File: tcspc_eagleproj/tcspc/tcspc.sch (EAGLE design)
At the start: 72 parts, among them U1 THS788, U2 MCP4725, U3 ADCMP582, U4 LT6003_SOT23-5, X1 SMA

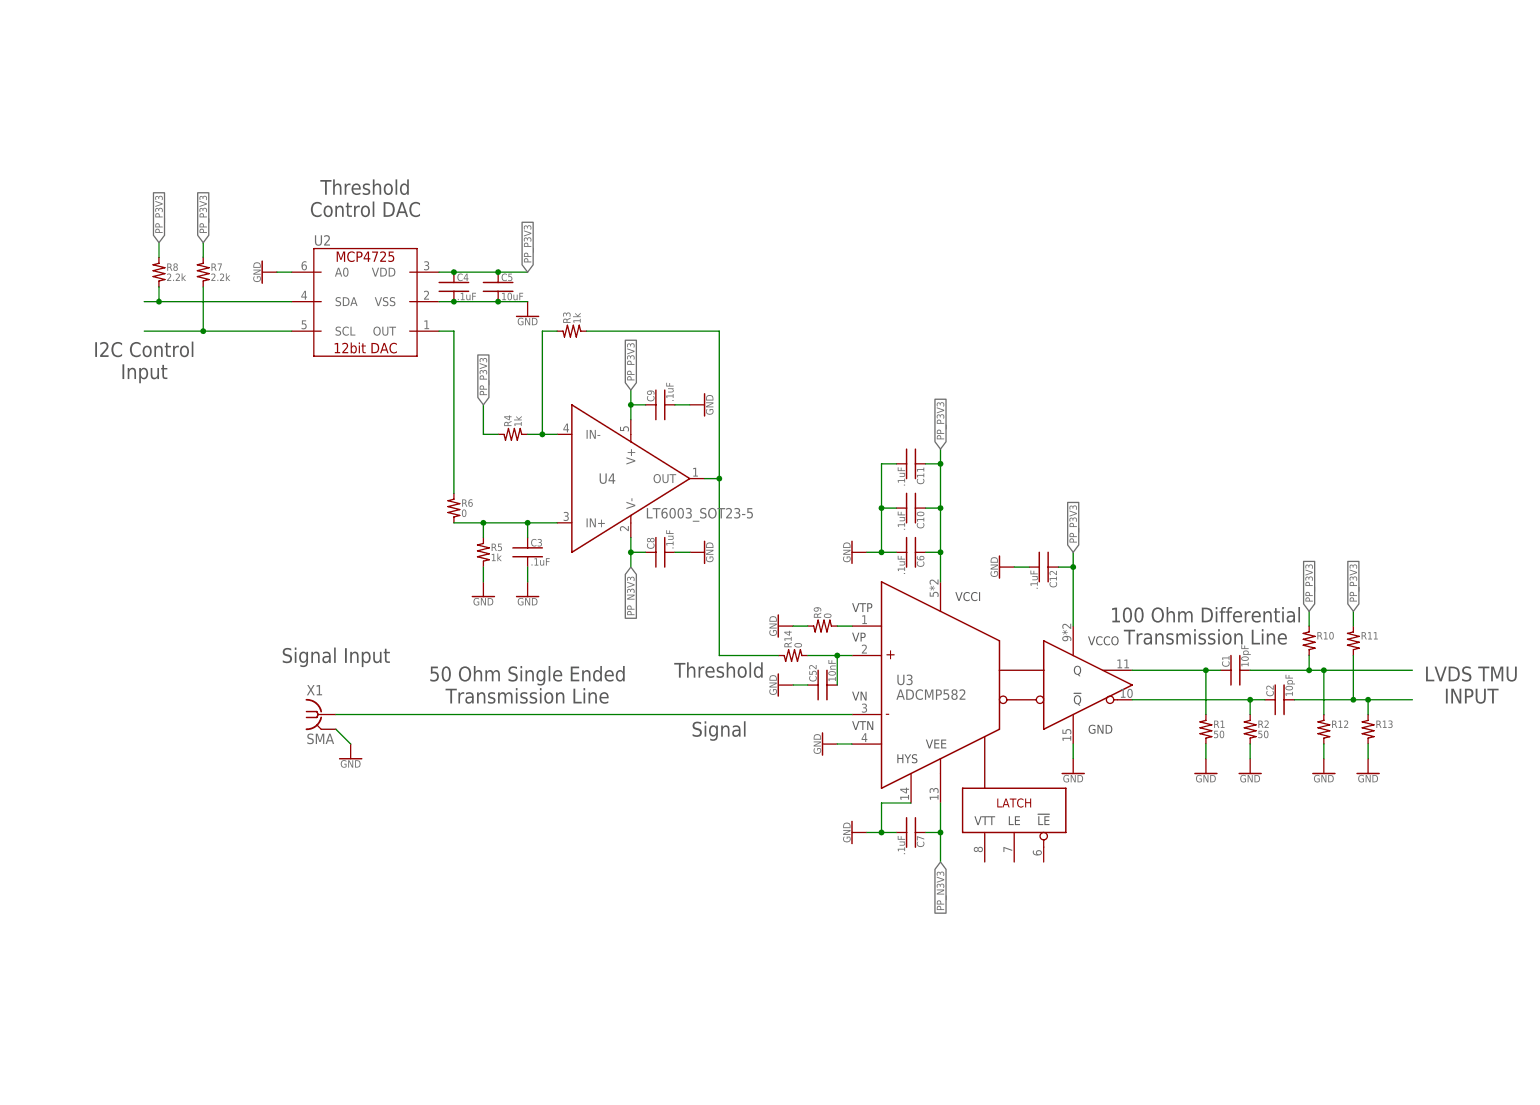
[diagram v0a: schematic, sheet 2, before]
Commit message: not 100% sure what changes got made here but there was a good chunk of progress nonetheless
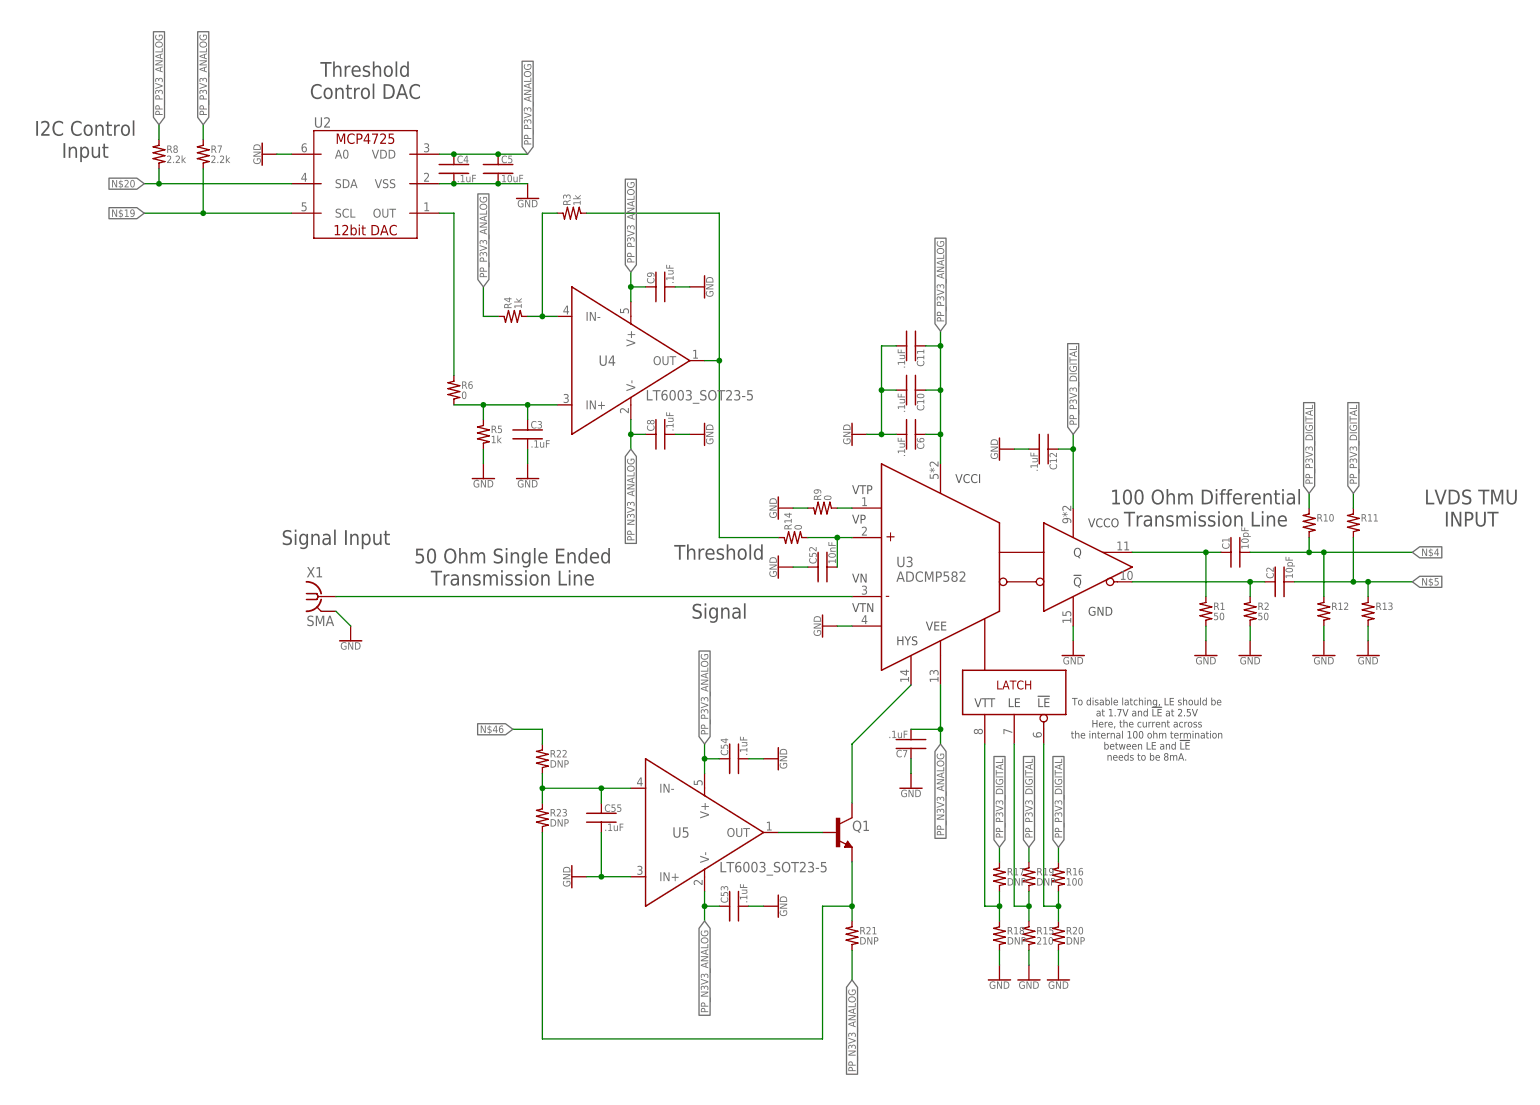
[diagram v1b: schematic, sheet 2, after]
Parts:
- added C53, C54, C55: .1uF, tcspc_lib:CAP_0402
- added Q1: (no value), jack_semi:BJT_NPN
- added R15: 210, tcspc_lib:RES_0402
- added R16: 100, tcspc_lib:RES_0402
- added R17, R18, R19, R20, R21, R22, R23: DNP, tcspc_lib:RES_0402
- added U5: LT6003_SOT23-5, tcspc_lib:LT6003_SOT23-5
- C3, C4, C5, C8, C9: device tcspc_lib:CAP_0603 -> tcspc_lib:CAP_0402
- R3, R4, R5, R6, R7, R8: device tcspc_lib:RES_0603 -> tcspc_lib:RES_0402
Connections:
- removed net PP_N3V3: C7.1, C8.1, U3.VEE, U4.V-
- new net N$38: R17.2, R18.1, U3.VTT
- new net N$39: R15.1, R19.2, U3.LE
- new net N$41: R16.2, R20.1, U3.!LE
- new net N$42: Q1.C, U3.HYS
- new net N$43: Q1.B, U5.OUT
- new net N$45: C55.1, R22.2, R23.1, U5.IN-
- new net N$46: R22.1
- new net N$47: Q1.E, R21.1, R23.2
- new net PP_N3V3_ANALOG: C53.1, C7.2, C8.1, R21.2, U3.VEE, U4.V-, U5.V-
- new net PP_P3V3_ANALOG: C10.1, C11.1, C4.1, C5.1, C54.1, C6.1, C9.1, R4.1, R7.1, R8.1, U2.VDD, U3.VCCI, U4.V+, U5.V+
- new net PP_P3V3_DIGITAL: C12.1, R10.1, R11.1, R16.1, R17.1, R19.1, U3.VCCO
- net GND: now also C53.2, C54.2, C55.2, C7.1, R15.2, R18.2, R20.2, U5.IN+; no longer C7.2, U3.HYS
- net PP_P3V3: no longer C10.1, C11.1, C12.1, C4.1, C5.1, C6.1, C9.1, R10.1, R11.1, R4.1, R7.1, R8.1, U2.VDD, U3.VCCI, U3.VCCO, U4.V+
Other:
- note added: "To disable latching, LE should be at 1.7V and !LE! at 2.5V Here, the current across the internal 100 ohm termination between LE and !LE! needs to be 8mA."
- moved on the sheet: C1, C10, C11, C12, C2, C3, C4, C5, C52, C6, C7, C8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
